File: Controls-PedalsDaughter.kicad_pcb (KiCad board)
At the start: 2 copper layers, 50.8 x 74.2 mm, 54 parts, among them J1 Brake Pos. Sensor, J2 Accel Pos. Sensor, J3 PeripheralCANConnector, J4 Conn_01x02, J5 PeripheralCANConnector, U1 RI3-1205S, U2 PeripheralSOM, U3 TLV9301xDCK, U4 TLV70130DBVR, U5 AMC1300BDWV, U6 TLV9301xDCK

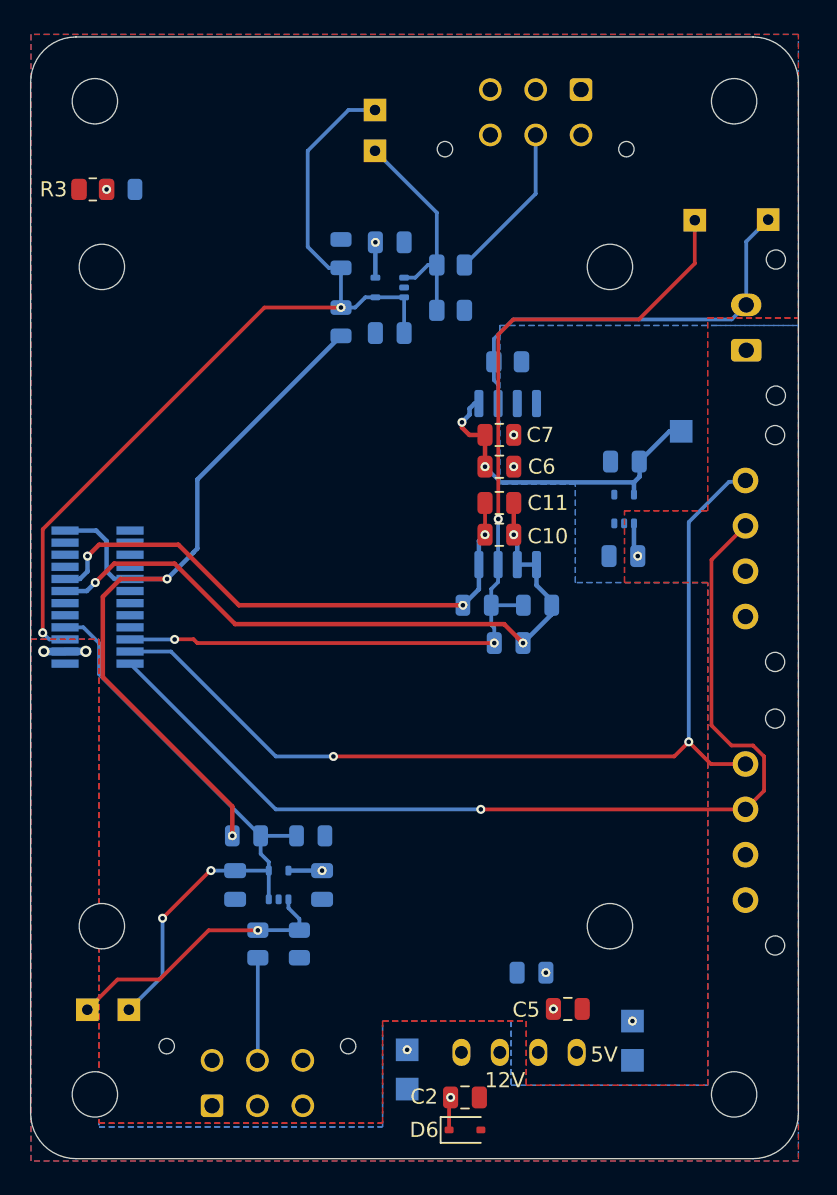
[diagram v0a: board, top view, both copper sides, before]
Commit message: Donesies?
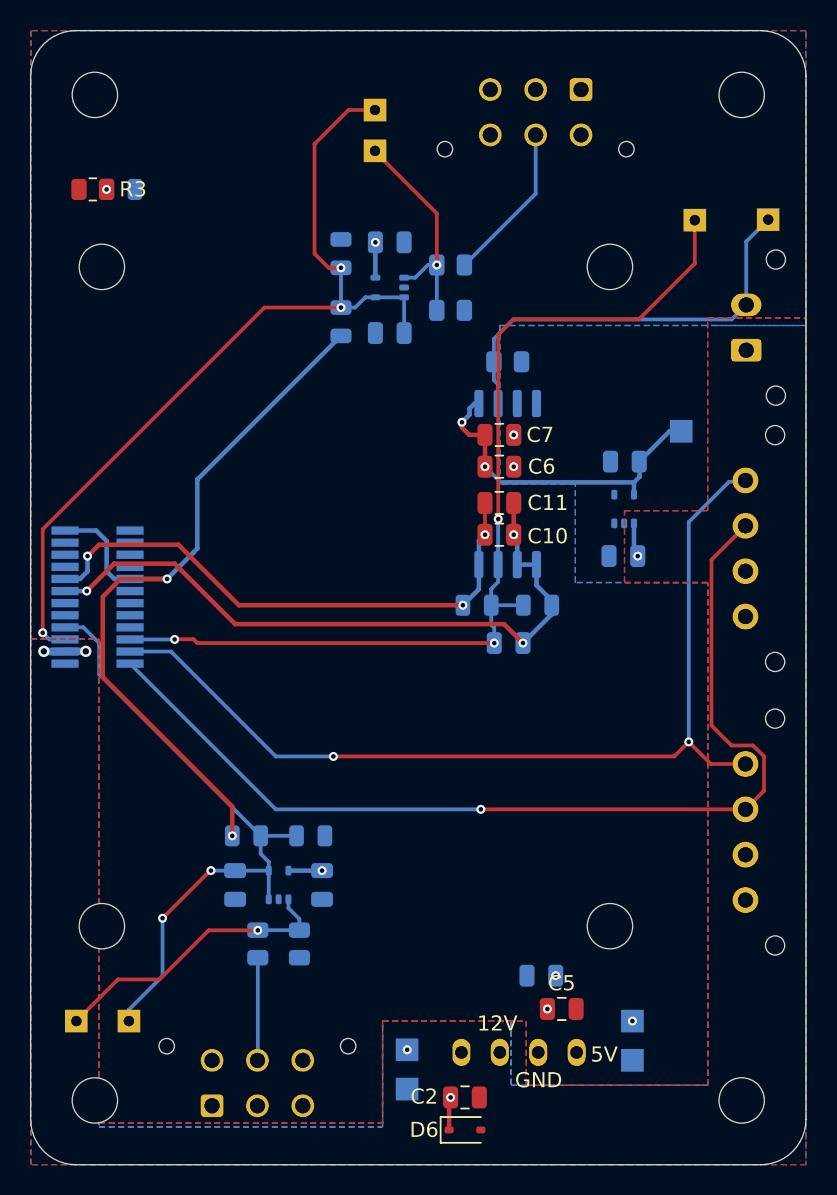
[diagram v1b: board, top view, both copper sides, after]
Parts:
- moved Accel_Raw 1.04 mm to (125.5, 128.0)
- moved Accel 0.75 mm to (129.0, 128.0)
- moved C4 0.68 mm to (156.2, 125.0)
- moved H2 0.65 mm to (172.8, 66.8)
- moved H3 0.64 mm to (172.8, 133.2)
- moved H1 0.42 mm to (130.0, 66.8)
- moved ? 0.40 mm to (130.0, 133.2)
- moved C5 0.40 mm to (157.6, 127.2)
- renumbered D7 to PWR
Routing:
- net Net-(U3-+): track 18.5 -> 19.6 mm
- net /Accel: track 42.0 -> 42.8 mm
- net /Brake_Pot: track 58.5 -> 58.1 mm, vias 2 -> 3
- net Net-(U6-+): vias 0 -> 1
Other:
- board size 50.8 x 74.2 mm -> 51.3 x 75 mm
- board text added: "GND"
